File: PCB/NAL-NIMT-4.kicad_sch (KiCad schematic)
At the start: 19 parts

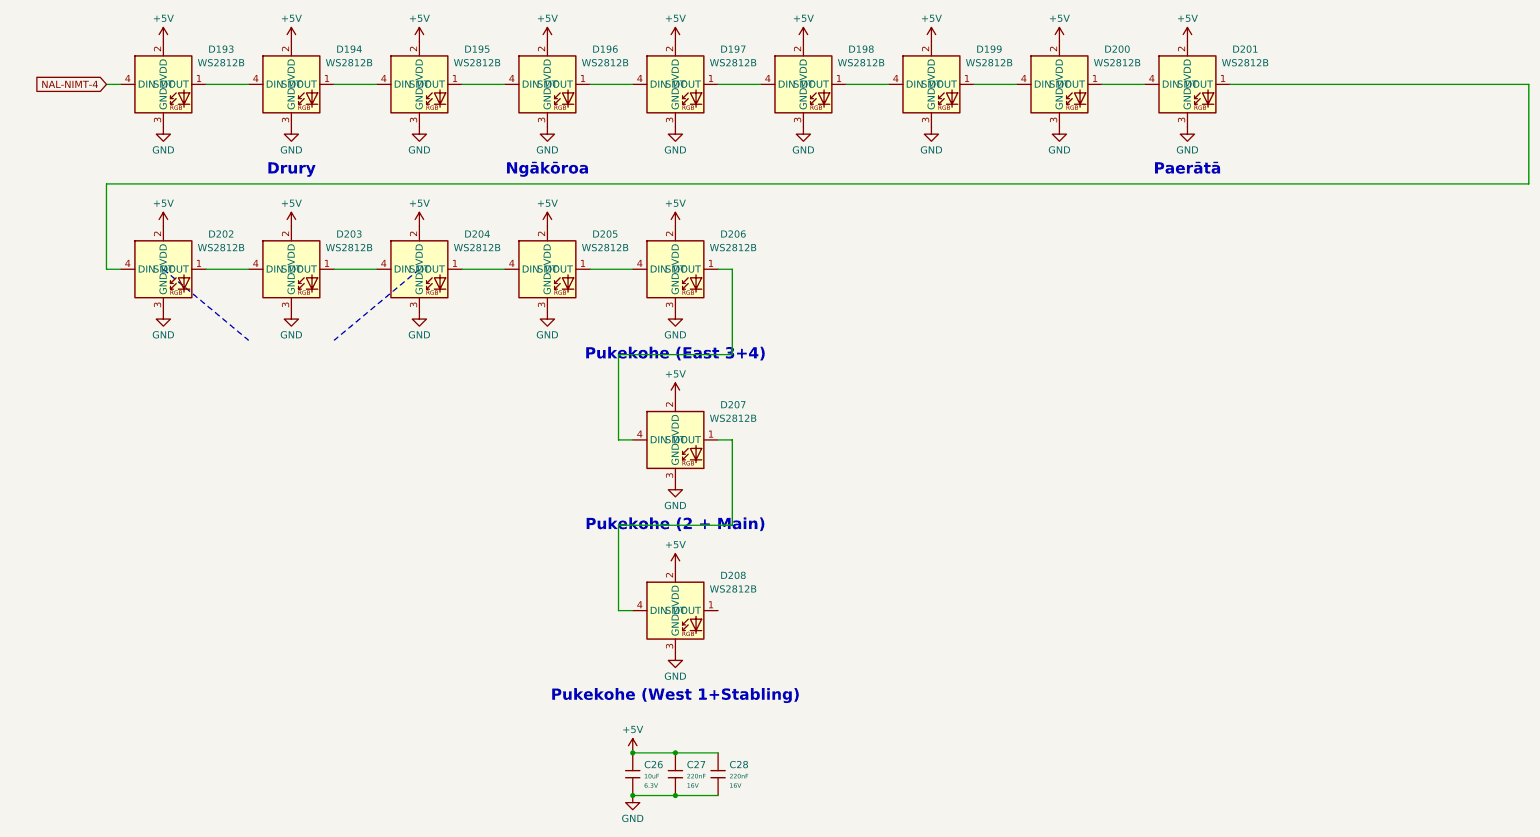
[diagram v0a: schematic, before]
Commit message: V1.1.0 PCB
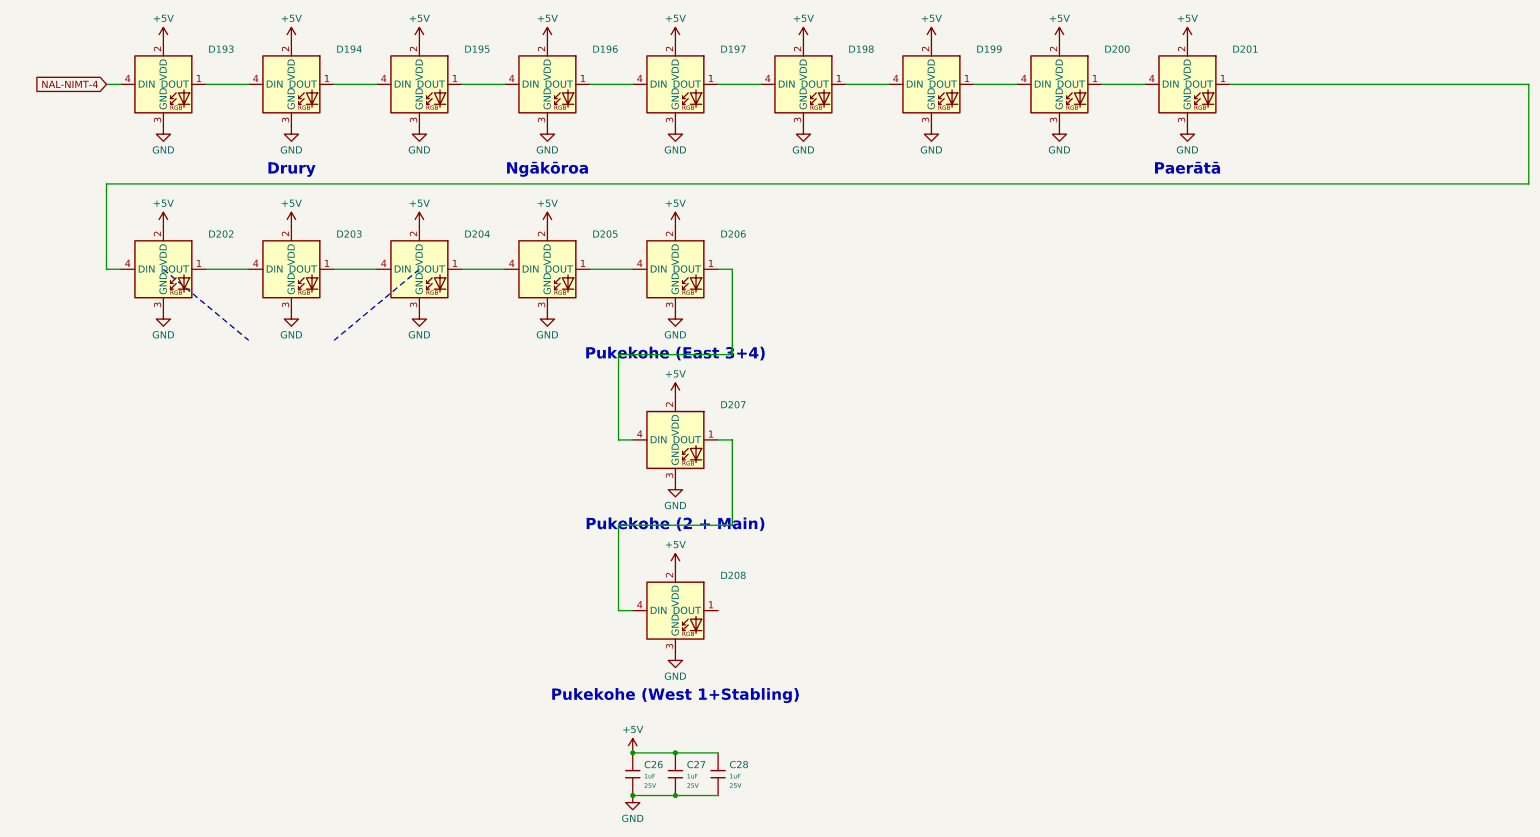
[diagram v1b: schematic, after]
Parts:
- C26: value 10uF -> 1uF; symbol PCM_JLCPCB-Capacitors:0402,10uF -> PCM_JLCPCB-Capacitors:0402,1uF; Capacitance 10uF -> 1uF; LCSC C15525 -> C52923; Part CL05A106MQ5NUNC -> CL05A105KA5NQNC; Price 0.007USD -> 0.006USD; Stock 1595146 -> 9606588; Tolerance ±20% -> ±10%; Voltage Rated 6.3V -> 25V
- C27, C28: value 220nF -> 1uF; symbol PCM_JLCPCB-Capacitors:0402,220nF -> PCM_JLCPCB-Capacitors:0402,1uF; Capacitance 220nF -> 1uF; LCSC C16772 -> C52923; Part CL05B224KO5NNNC -> CL05A105KA5NQNC; Price 0.008USD -> 0.006USD; Stock 351761 -> 9606588; Temperature Coefficient X7R -> X5R; Voltage Rated 16V -> 25V
- D193, D194, D195, D196, D197, D198, D199, D200, D201, D202, D203, D204, D205, D206, D207, D208: value WS2812B -> XL-1615RGBC-WS2812B-S; LCSC C5349954 -> C41413180; Manufacturer XINGLIGHT -> (none); Part XL-1615RGBC-WS2812B -> (none); Process SMT -> (none)

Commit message: Update to meet OSHWA Certification
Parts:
- D193, D194, D195, D196, D197, D198, D199, D200, D201, D202, D203, D204, D205, D206, D207, D208: Manufacturer (none) -> XINGLIGHT; Part (none) -> XL-1615RGBC-WS2812B-S
